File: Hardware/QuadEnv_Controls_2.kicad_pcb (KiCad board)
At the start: 2 copper layers, 18.8 x 110 mm, 15 parts, among them J1 Conn_01x08, J2 Conn_01x04, J3 Conn_01x05, J4 Conn_01x04, J5 Gate_In, J6 Env_Out

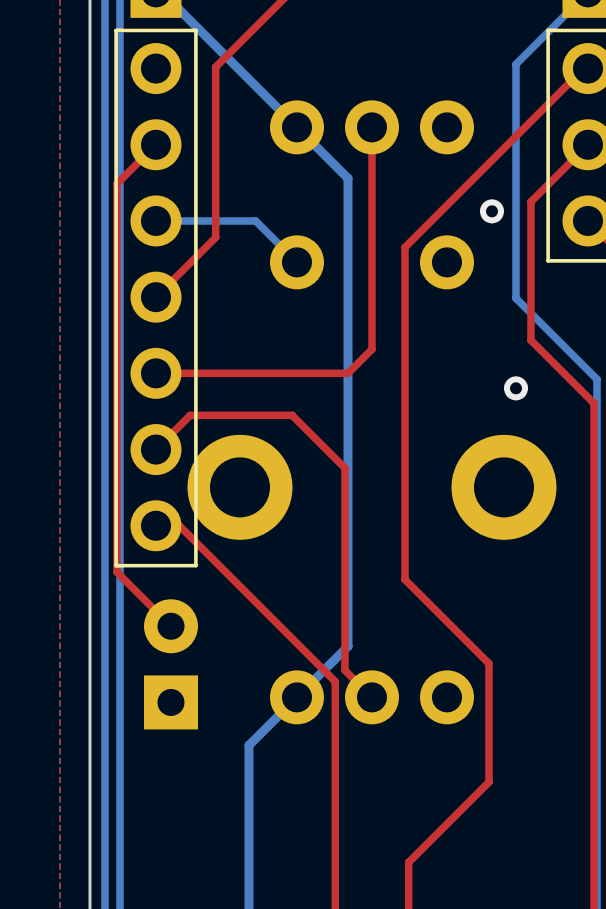
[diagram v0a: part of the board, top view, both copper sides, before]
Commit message: Completed v2 design
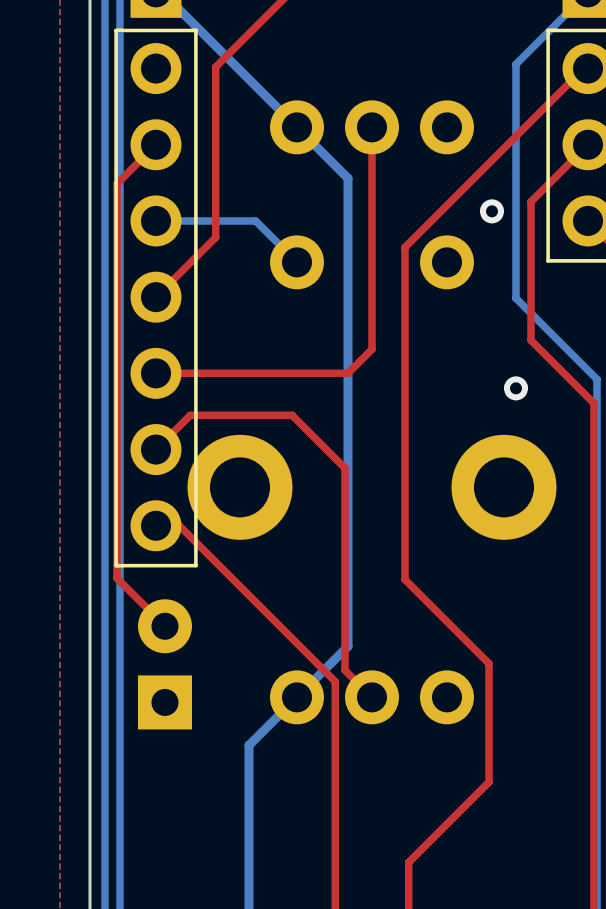
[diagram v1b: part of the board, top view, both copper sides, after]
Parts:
- moved D5 0.20 mm to (52.5, 97.4)
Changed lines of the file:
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@@
   )
   (footprint "Custom_Footprints:LED_D3.0mm" (layer "B.Cu")
-    (at 52.7 97.4 90)
+    (at 52.5 97.4 90)
     (descr "LED, diameter 3.0mm, 2 pins")
     (tags "LED diameter 3.0mm 2 pins")
@@
   (segment (start 64.2 143.7) (end 63.5 143) (width 0.25) (layer "F.Cu") (net 18))
   (segment (start 64.2 151.72) (end 64.2 143.7) (width 0.25) (layer "F.Cu") (net 18))
-  (segment (start 50.9 94.33) (end 50.9 81.38) (width 0.25) (layer "F.Cu") (net 27))
   (segment (start 50.9 81.38) (end 52.2 80.08) (width 0.25) (layer "F.Cu") (net 27))
-  (segment (start 52.7 96.13) (end 50.9 94.33) (width 0.25) (layer "F.Cu") (net 27))
+  (segment (start 50.9 94.53) (end 50.9 81.38) (width 0.25) (layer "F.Cu") (net 27))
+  (segment (start 52.5 96.13) (end 50.9 94.53) (width 0.25) (layer "F.Cu") (net 27))
   (segment (start 56.9 84) (end 55.52 82.62) (width 0.25) (layer "B.Cu") (net 28))
   (segment (start 55.52 82.62) (end 52.2 82.62) (width 0.25) (layer "B.Cu") (net 28))
